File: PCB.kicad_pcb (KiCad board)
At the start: 2 copper layers, 60 x 60 mm, 52 parts, among them J1 USB_C_Receptacle_USB2.0_16P, J10 Conn_01x06_Socket, J11 Conn_01x02_Pin, J13 Conn_01x05_Pin, J2 Conn_01x06_Socket, J3 Conn_01x04_Pin, J4 Conn_01x05_Pin, J5 Conn_01x02_Pin, J6 Conn_01x02_Pin, J7 Conn_01x02_Pin, J8 Conn_01x04_Pin, J9 Conn_01x05_Pin, SW1 SW_Push, SW2 SW_Push, U1 TMC2209_SILENTSTEPSTICK, U2 USBLC6-2SC6, U4 AMS1117-3.3 (UMW), U5 TMC2209_SILENTSTEPSTICK, U6 ESP32-S3-WROOM-1

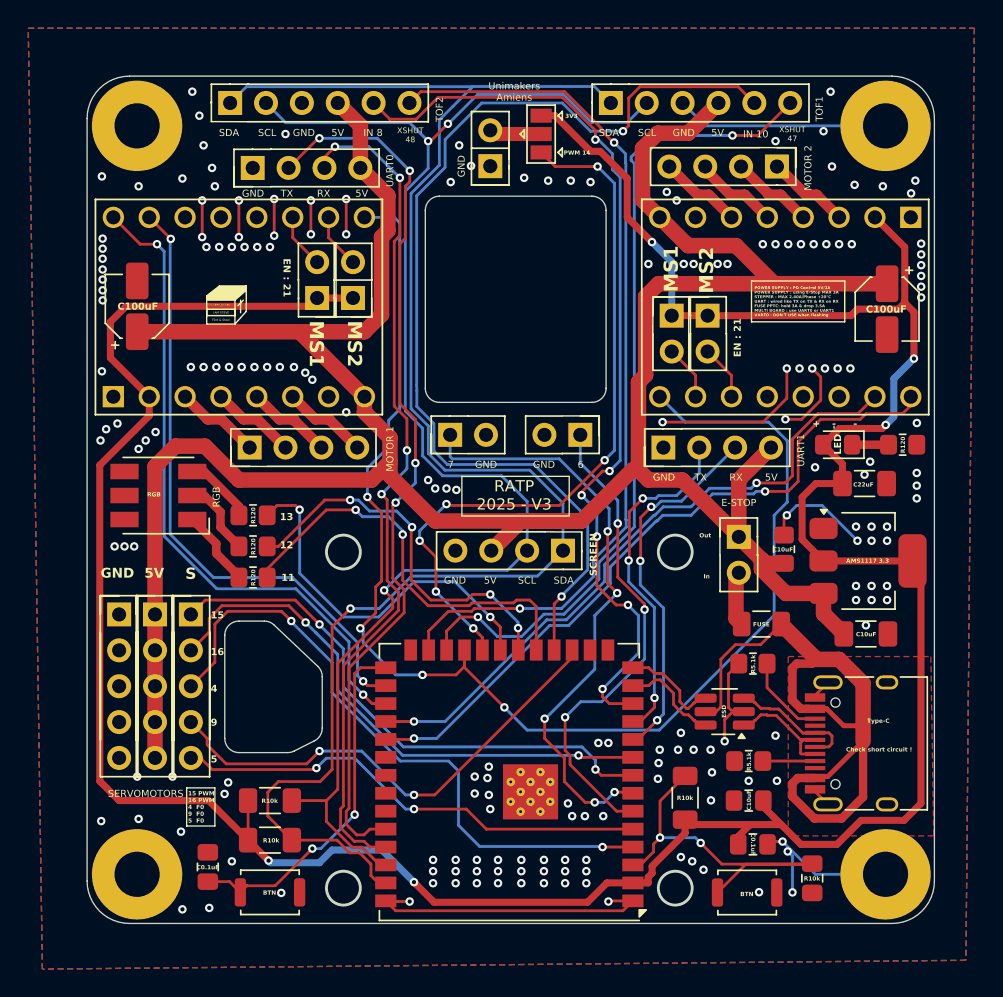
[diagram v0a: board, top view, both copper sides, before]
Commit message: V3 Corrigée (ToF)
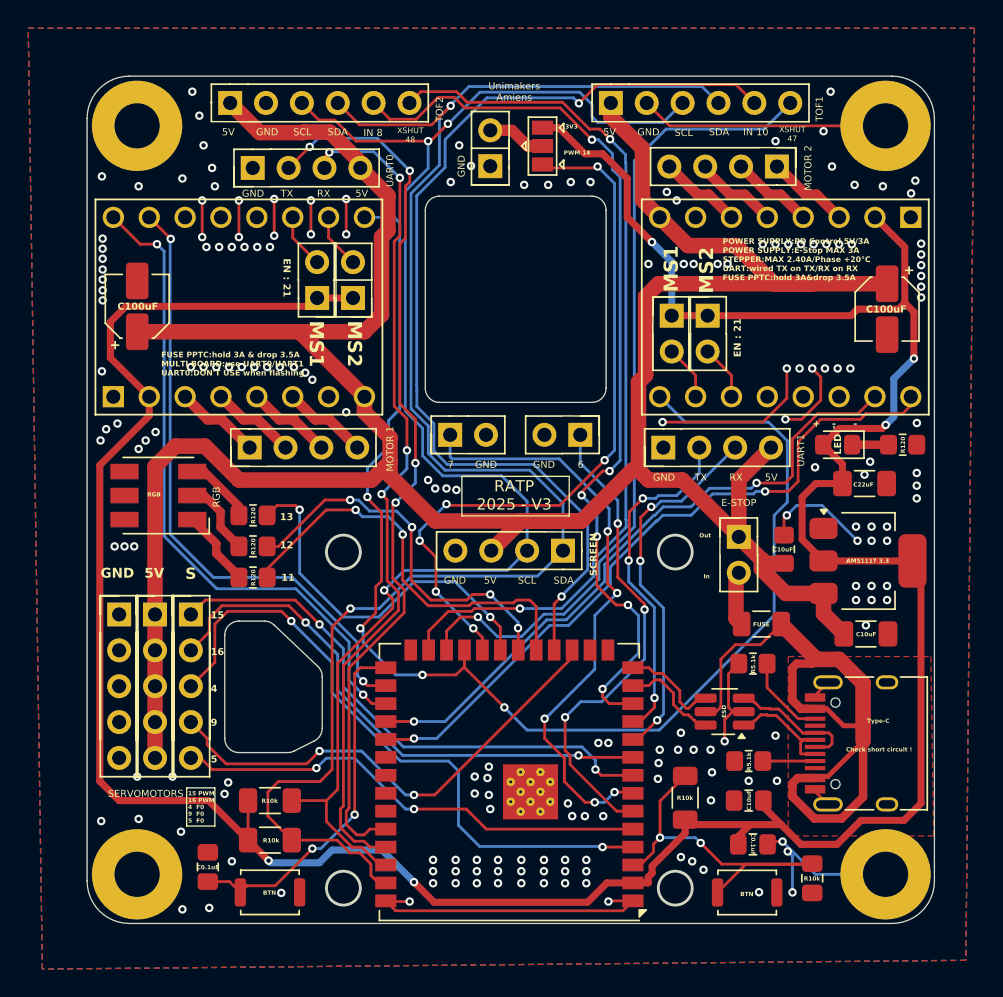
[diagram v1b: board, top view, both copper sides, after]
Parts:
- C7: value 22uF -> 10uF
- moved JP5 0.86 mm to (145.5, 76.5)
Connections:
- J10 pad 1: SDA -> VCC_5V
- J10 pad 2: SCL -> GND
- J10 pad 3: GND -> SCL
- J10 pad 4: VCC_5V -> SDA
- J2 pad 1: SDA -> VCC_5V
- J2 pad 2: SCL -> GND
- J2 pad 3: GND -> SCL
- J2 pad 4: VCC_5V -> SDA
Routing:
- net VCC_5V: track 198.9 -> 202.4 mm
- net GND: track 97.8 -> 100.4 mm, vias 192 -> 191
- net GPIO10: track 73.3 -> 71.0 mm
- net Net-(J11-Pin_2): track 3.71 -> 4.54 mm
- net SDA: track 117.0 -> 116.3 mm, vias 1 -> 2
- net XSHUT1: track 58.7 -> 58.2 mm, vias 2 -> 1
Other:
- board text added: "FUSE PPTC:hold 3A & drop 3.5A MULTI BOARD:use UART0/UART1 UART0:DON'T USE when flashing"
- board text added: "POWER SUPPLY:PD Control 5V/3A POWER SUPPLY:E-Stop MAX 3A STEPPER:MAX 2.40A/Phase +20°C UART:wired TX on TX/RX on RX FUSE PPTC:hold 3A&drop 3.5A"
- board text removed: "Chicken Jockey"
- board text removed: "Flint & Steel"
- board text removed: "I AM STEVE"
- board text removed: "POWER SUPPLY : PD Control 5V/3A POWER SUPPLY : using E-Stop MAX 3A STEPPER : MAX 2.40A/Phase +20°C UART : wired like TX on TX & RX on RX FUSE PPTC: hold 3A & drop 3.5A MULTI BOARD : use UART0 or UART1 UART0 : DON'T USE when flashing"
